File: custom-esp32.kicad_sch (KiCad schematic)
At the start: 26 parts, among them J3 USB_C_Receptacle_USB2.0_16P, U1 ESD7104MUTAG, U2 ENS210, U3 ESP32-S3-MINI-1-N8, U4 TLV75801PDRV

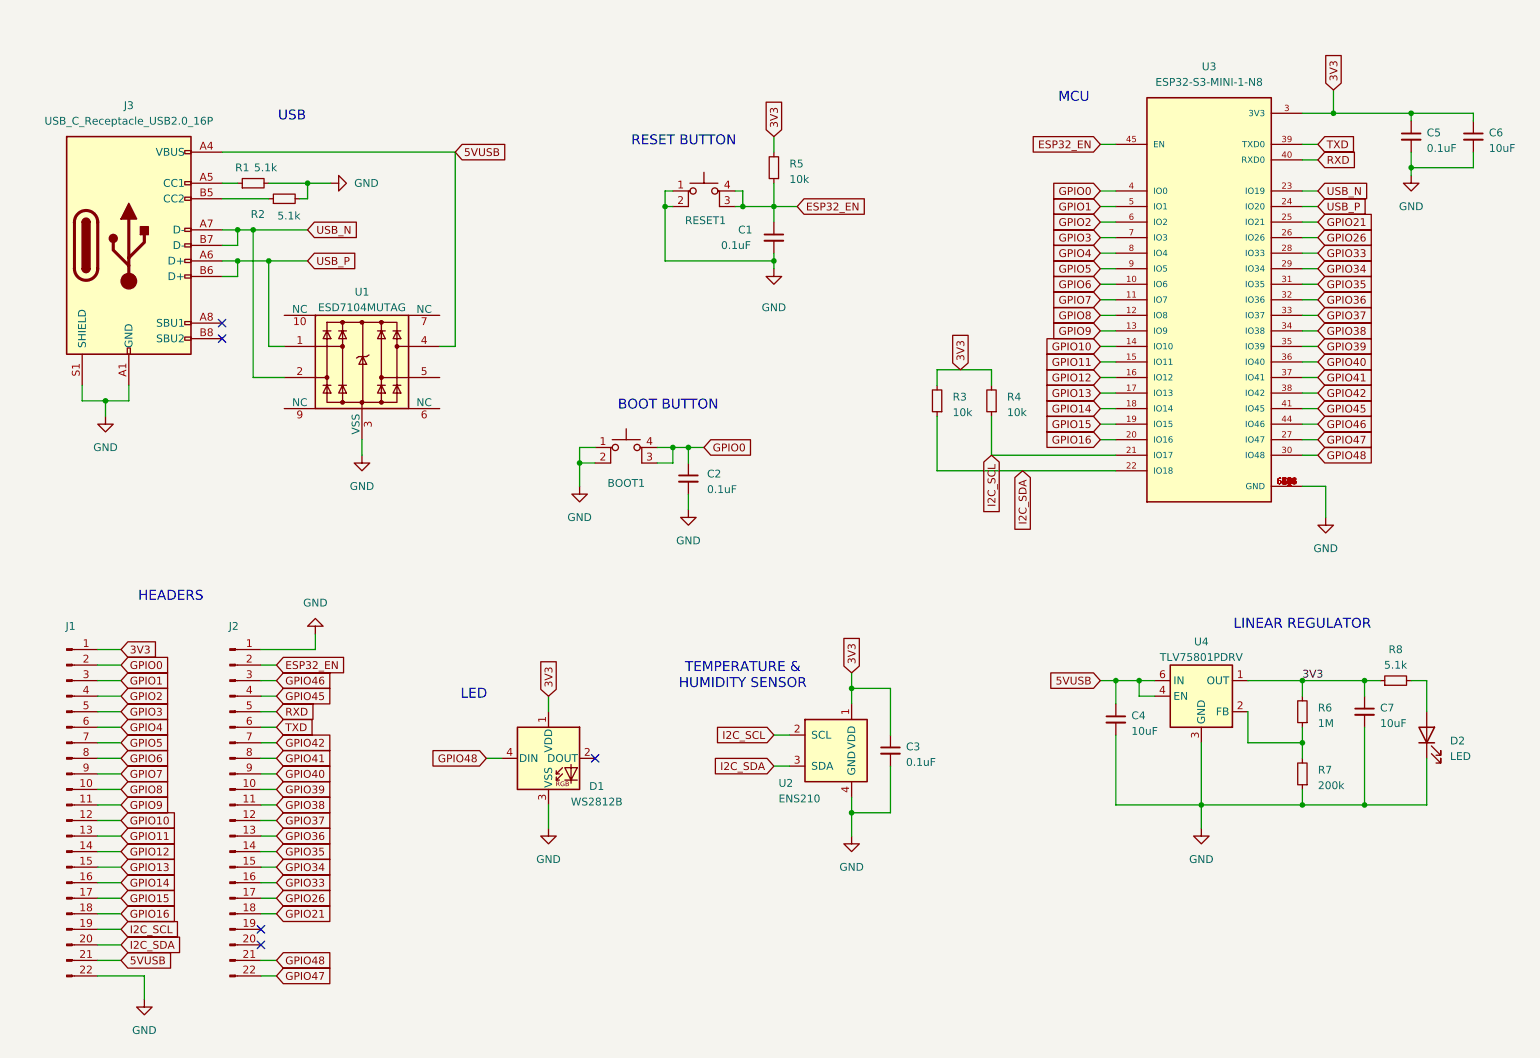
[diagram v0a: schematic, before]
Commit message: Update schematic
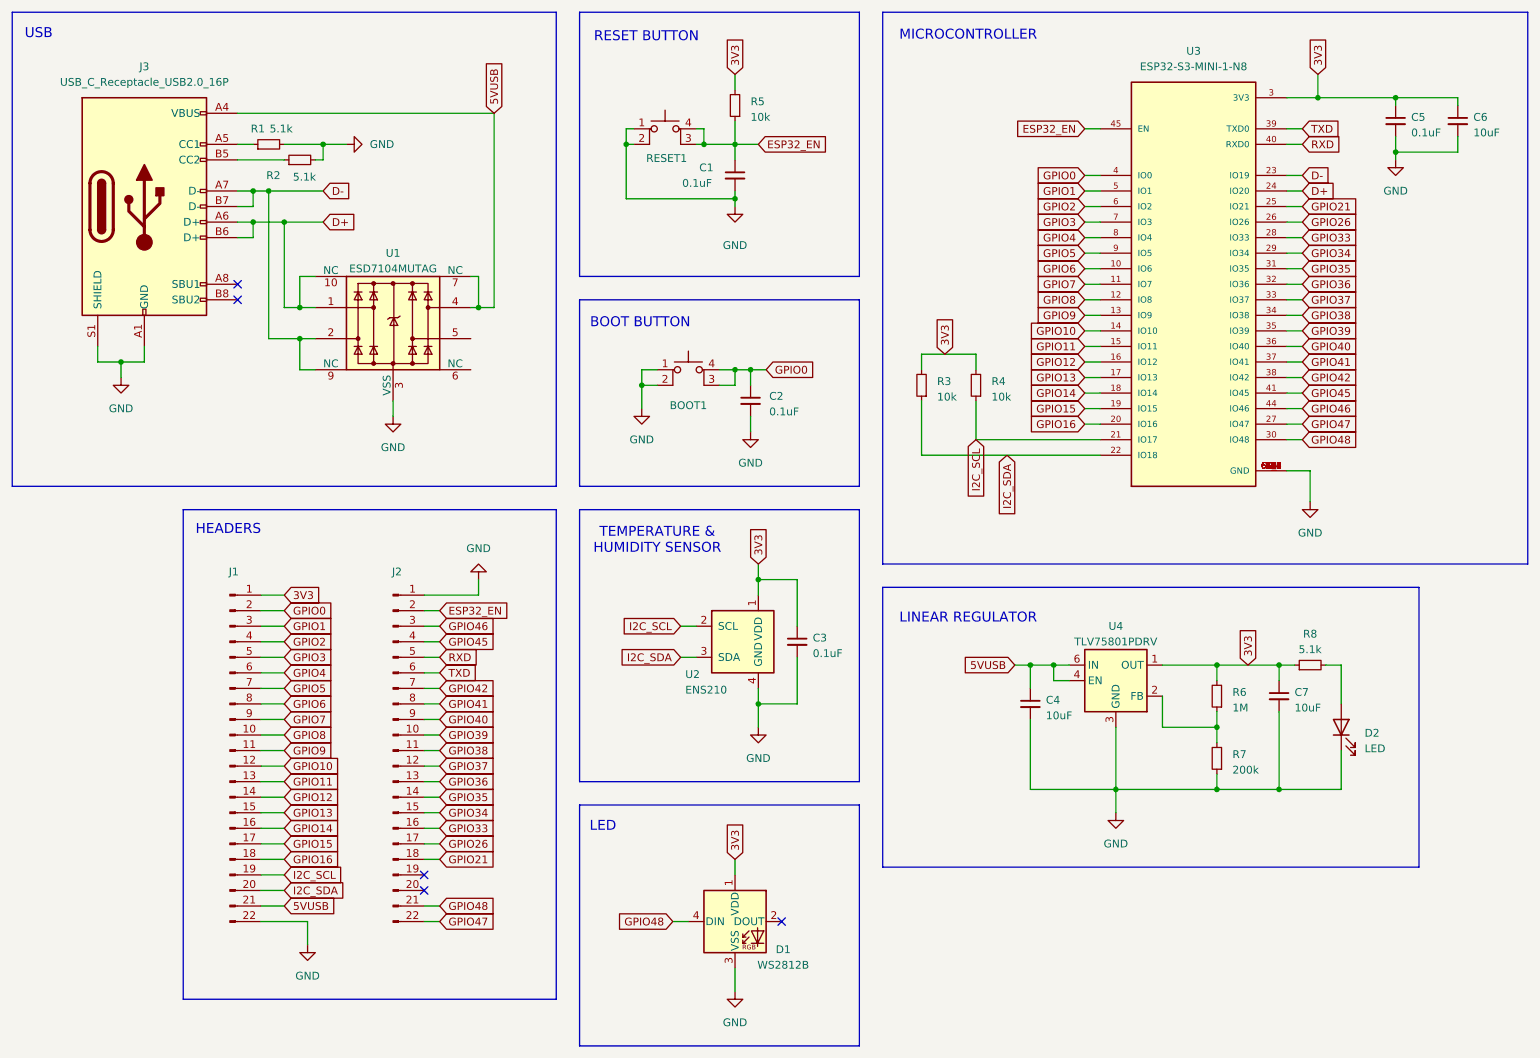
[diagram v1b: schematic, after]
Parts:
- U3: footprint ESP32-S3-MINI-1-N8:XCVR_ESP32-S3-MINI-1-N8 -> ESP32_S3_MINI_1_N8:XCVR_ESP32-S3-MINI-1-N8
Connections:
- net USB_N is gone; now on net D-: J3.A7 (D-), J3.B7 (D-), U1.2, U3.23 (IO19)
- net USB_P is gone; now on net D+: J3.A6 (D+), J3.B6 (D+), U1.1, U3.24 (IO20)
- net 5VUSB: now also U1.7 (NC)
- net D+: now reaches U1.10 (NC)
- net D-: now reaches U1.9 (NC)
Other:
- note added: "MICROCONTROLLER"
- note removed: "MCU"
- title: (none) -> Custom EPS32
- moved on the sheet: BOOT1, C1, C2, C3, C4, C5, C6, C7, D1, D2, J1, J2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
